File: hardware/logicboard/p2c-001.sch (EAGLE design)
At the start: 45 parts, among them IC1 74LS07N, K1 G5V1, T1 2SC1815

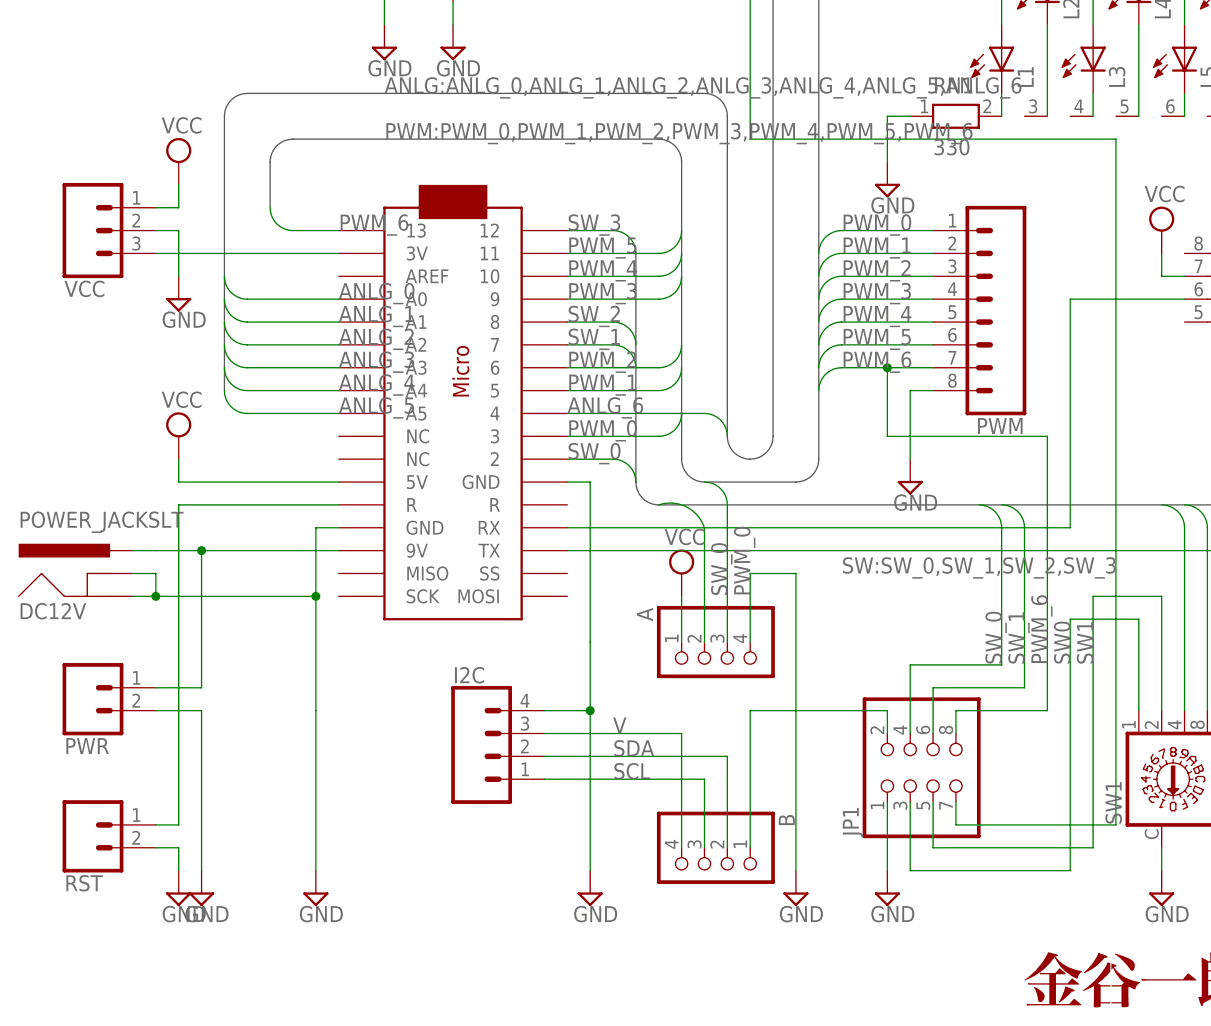
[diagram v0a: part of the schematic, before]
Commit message: Pinhead.
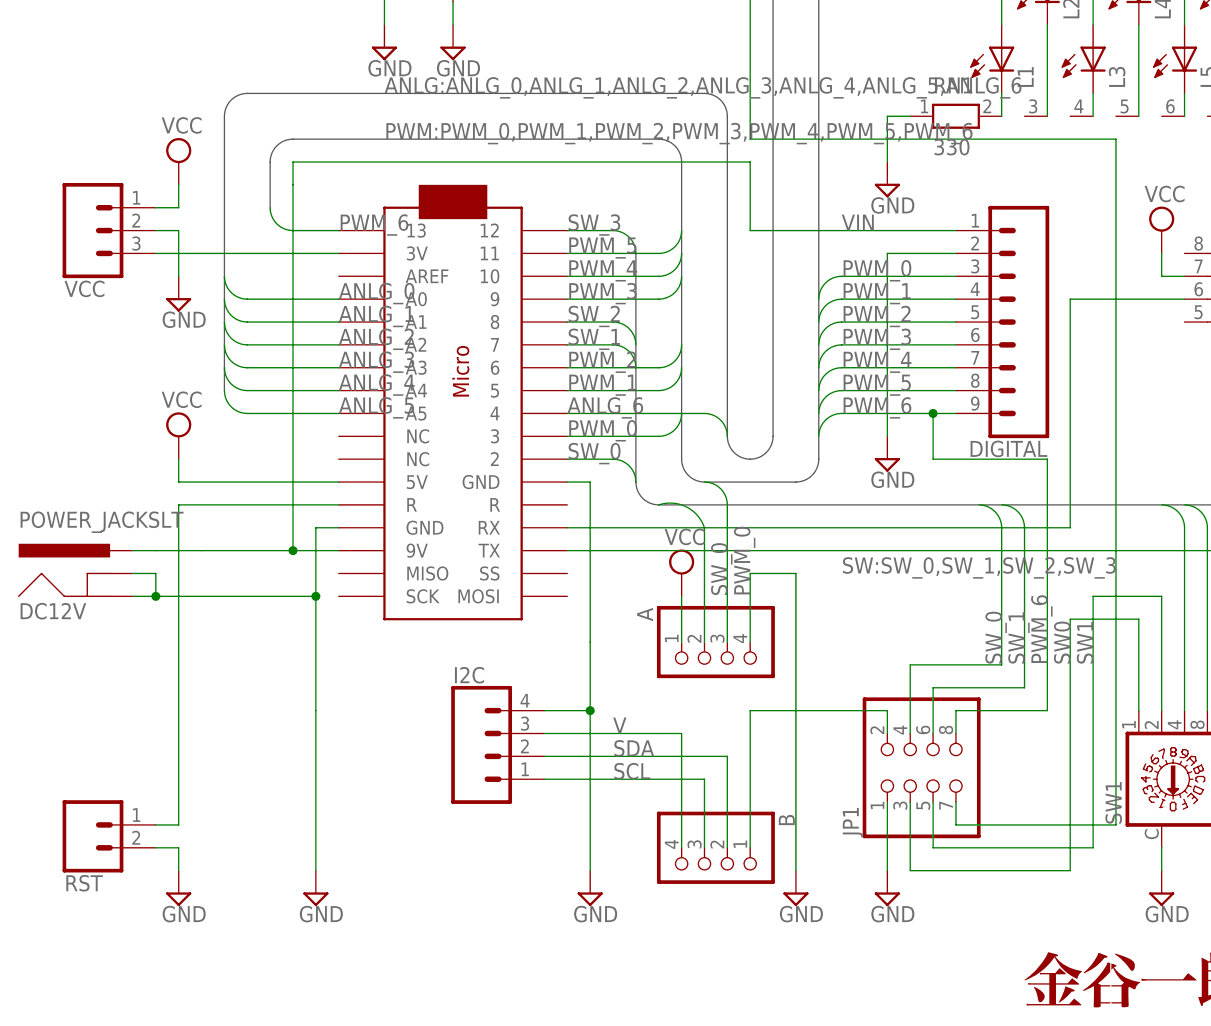
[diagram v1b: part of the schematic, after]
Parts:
- removed PWM: (no value), SparkFun-Connectors:CONN_08"
- removed PWR: (no value), SparkFun-Connectors:CONN_02
- added DIGITAL: (no value), SparkFun-Connectors:CONN_09
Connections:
- net GND: now also DIGITAL.2; no longer PWM.8, PWR.2
- net PWM_0: now also DIGITAL.3; no longer PWM.1
- net PWM_1: now also DIGITAL.4; no longer PWM.2
- net PWM_2: now also DIGITAL.5; no longer PWM.3
- net PWM_3: now also DIGITAL.6; no longer PWM.4
- net PWM_4: now also DIGITAL.7; no longer PWM.5
- net PWM_5: now also DIGITAL.8; no longer PWM.6
- net PWM_6: now also DIGITAL.9; no longer PWM.7
- net VIN: now also DIGITAL.1; no longer PWR.1
